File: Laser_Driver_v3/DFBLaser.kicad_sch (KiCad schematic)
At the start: 30 parts, among them Q15 IRLML6344TRPBF, Q16 IRLML6344TRPBF, U23 OPA192IDR, U24 OPA192IDR

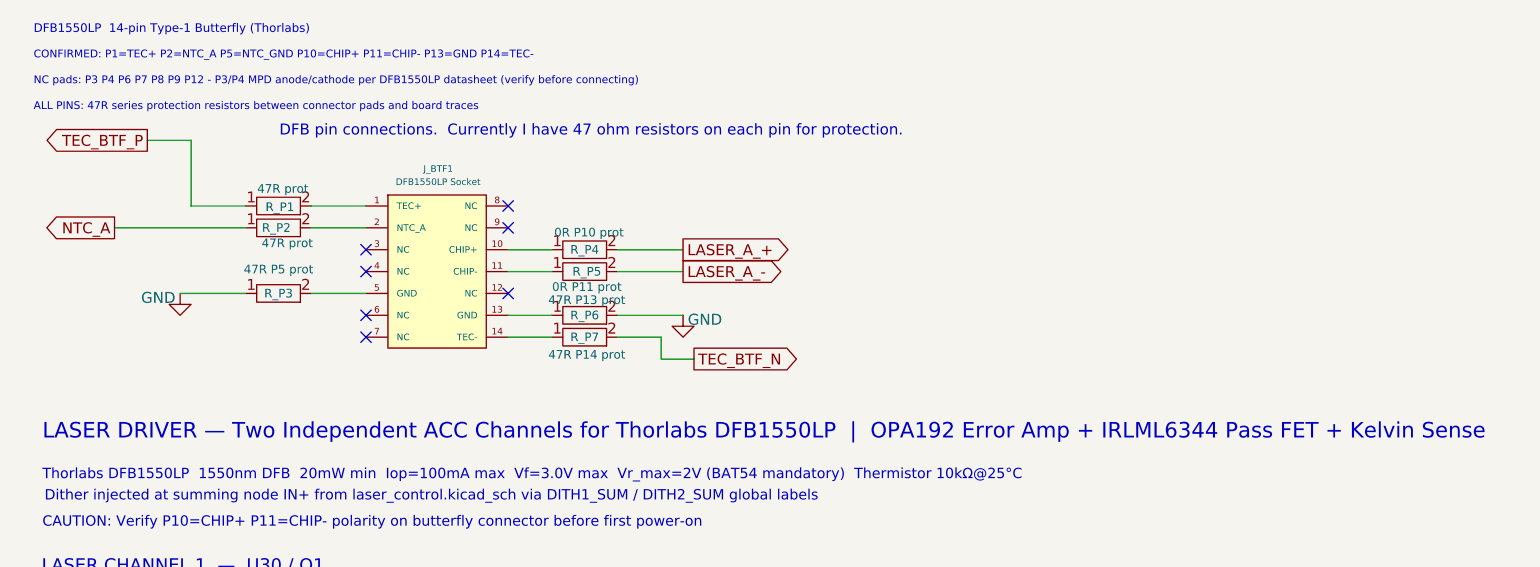
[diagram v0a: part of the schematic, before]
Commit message: first placement of all components on pcb.
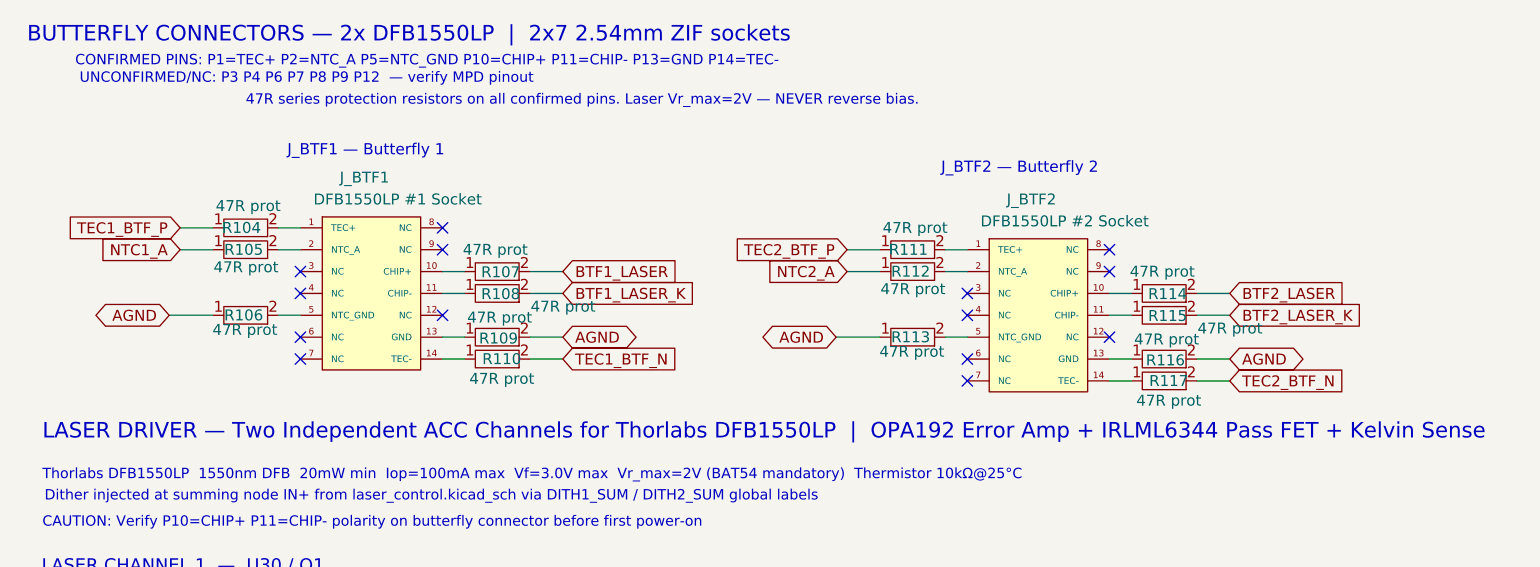
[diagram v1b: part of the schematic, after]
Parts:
- removed R_P1, R_P2: 47R prot, Resistor_SMD:R_0805_2012Metric_Pad1.20x1.40mm_HandSolder, symbol Device:R
- removed R_P3: 47R P5 prot, Resistor_SMD:R_0805_2012Metric_Pad1.20x1.40mm_HandSolder, symbol Device:R
- removed R_P4: 0R P10 prot, Resistor_SMD:R_0805_2012Metric_Pad1.20x1.40mm_HandSolder, symbol Device:R
- removed R_P5: 0R P11 prot, Resistor_SMD:R_0805_2012Metric_Pad1.20x1.40mm_HandSolder, symbol Device:R
- removed R_P6: 47R P13 prot, Resistor_SMD:R_0805_2012Metric_Pad1.20x1.40mm_HandSolder, symbol Device:R
- removed R_P7: 47R P14 prot, Resistor_SMD:R_0805_2012Metric_Pad1.20x1.40mm_HandSolder, symbol Device:R
- added J_BTF2: DFB1550LP #2 Socket, Connector_PinSocket_2.54mm:PinSocket_2x07_P2.54mm_Vertical, symbol Connector:Conn_02x07_Odd_Even
- added R104, R105, R106, R107, R108, R109, R110, R111, R112, R113, R114, R115, R116, R117: 47R prot, Resistor_SMD:R_0805_2012Metric_Pad1.20x1.40mm_HandSolder, symbol Device:R
- J_BTF1: value DFB1550LP Socket -> DFB1550LP #1 Socket
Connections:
- net at J_BTF1.1 (TEC+): now also R104.2
- net at J_BTF1.13 (GND): now also R109.1
- net at J_BTF1.2 (NTC_A): now also R105.2
- net at J_BTF1.10 (CHIP+): now also R107.1
- net at J_BTF1.11 (CHIP-): now also R108.1
- net at J_BTF1.14 (TEC-): now also R110.1
- net at J_BTF1.5 (NTC_GND): now also R106.2
- new net: J_BTF2.5 (NTC_GND), R113.2
- new net: J_BTF2.14 (TEC-), R117.1
- new net: J_BTF2.1 (TEC+), R111.2
- new net: J_BTF2.13 (GND), R116.1
- new net: J_BTF2.2 (NTC_A), R112.2
- new net: J_BTF2.11 (CHIP-), R115.1
- new net: J_BTF2.10 (CHIP+), R114.1
- new net AGND: R106.1, R109.2, R113.1, R116.2
- new net BTF1_LASER: R107.2
- new net BTF1_LASER_K: R108.2
- new net BTF2_LASER: R114.2
- new net BTF2_LASER_K: R115.2
- new net NTC1_A: R105.1
- new net NTC2_A: R112.1
- new net TEC1_BTF_N: R110.2
- new net TEC1_BTF_P: R104.1
- new net TEC2_BTF_N: R117.2
- new net TEC2_BTF_P: R111.1
- no-connect marks 7 -> 14
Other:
- note added: "47R series protection resistors on all confirmed pins. Laser Vr_max=2V — NEVER reverse bias."
- note added: "BUTTERFLY CONNECTORS — 2x DFB1550LP | 2x7 2.54mm ZIF sockets"
- note added: "CONFIRMED PINS: P1=TEC+ P2=NTC_A P5=NTC_GND P10=CHIP+ P11=CHIP- P13=GND P14=TEC-"
- note added: "J_BTF1 — Butterfly 1"
- note added: "J_BTF2 — Butterfly 2"
- note added: "UNCONFIRMED/NC: P3 P4 P6 P7 P8 P9 P12 — verify MPD pinout"
- note removed: "ALL PINS: 47R series protection resistors between connector pads and board traces"
- note removed: "CONFIRMED: P1=TEC+ P2=NTC_A P5=NTC_GND P10=CHIP+ P11=CHIP- P13=GND P14=TEC-"
- note removed: "DFB pin connections. Currently I have 47 ohm resistors on each pin for protection."
- note removed: "DFB1550LP 14-pin Type-1 Butterfly (Thorlabs)"
- note removed: "NC pads: P3 P4 P6 P7 P8 P9 P12 - P3/P4 MPD anode/cathode per DFB1550LP datasheet (verify before connecting)"
